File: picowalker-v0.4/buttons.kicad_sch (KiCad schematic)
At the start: 0 parts

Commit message: v0.4: schematic laid out first draft
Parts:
- added C17, C18, C19: 0.1u, Capacitor_SMD:C_0402_1005Metric, symbol Device:C
- added R10, R11, R9: 5.1k, Resistor_SMD:R_0402_1005Metric, symbol Device:R
- added R12, R13, R14: 1k, Resistor_SMD:R_0402_1005Metric, symbol Device:R
- added SW3: BUT_R, symbol Switch:SW_Push
- added SW4: BUT_M, symbol Switch:SW_Push
- added SW5: BUT_L, symbol Switch:SW_Push
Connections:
- new net +3.3V: R10.2, R11.2, R9.2
- new net BUT.L: C19.1, R14.1
- new net BUT.M: C18.1, R13.1
- new net BUT.R: C17.1, R12.1
- new net BUT_L_1: R11.1, R14.2, SW5.2
- new net BUT_M_1: R10.1, R13.2, SW4.2
- new net BUT_R_1: R12.2, R9.1, SW3.2
- new net GND: C17.2, C18.2, C19.2, SW3.1, SW4.1, SW5.1
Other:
- note added: "Press resistor"
- note added: "Release resistor"

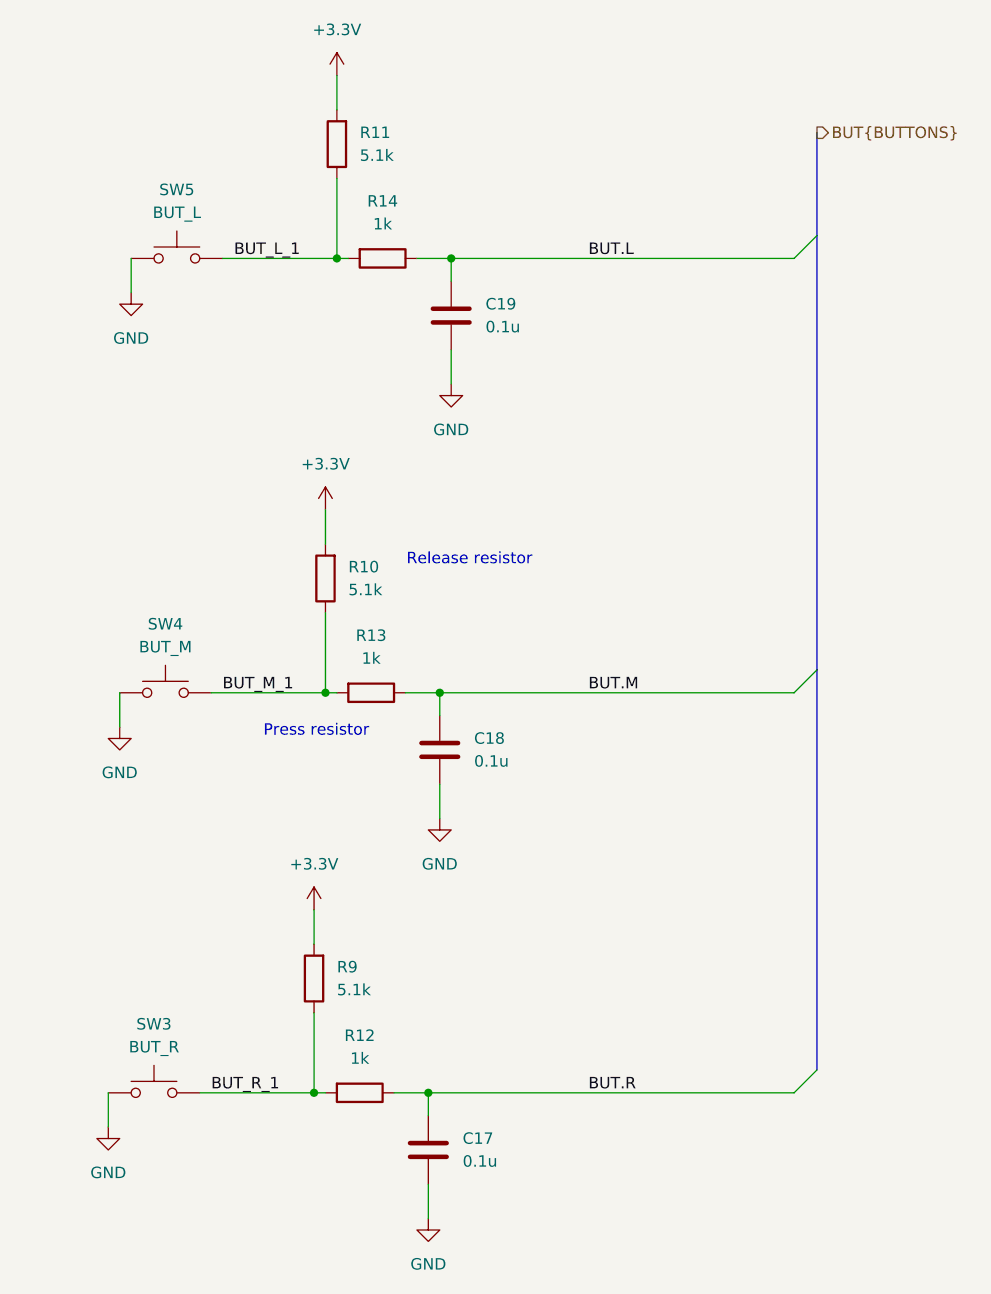
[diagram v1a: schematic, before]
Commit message: v0.4: first rough placement of PCB
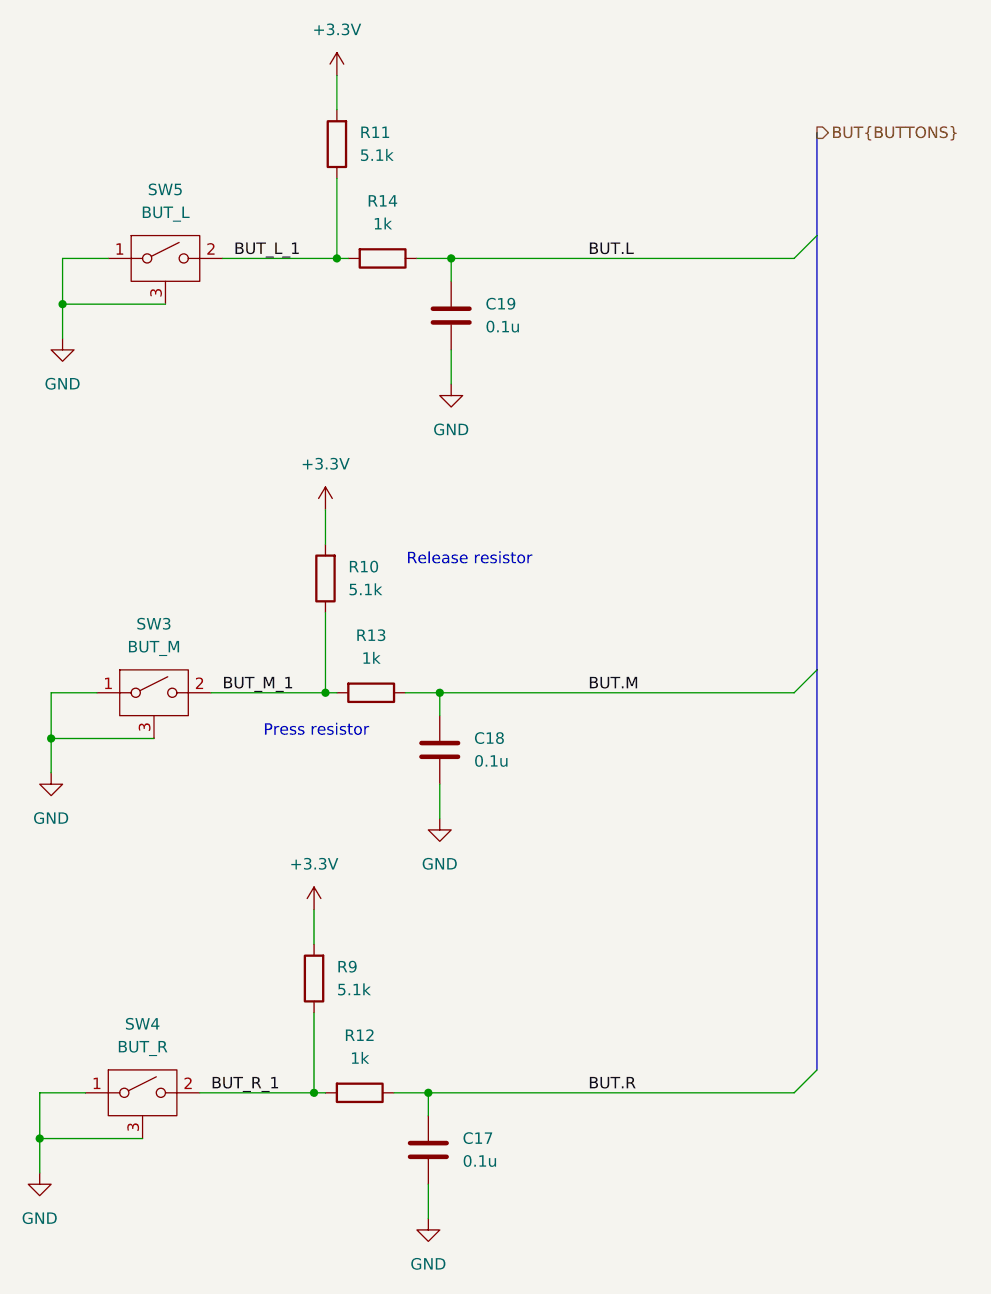
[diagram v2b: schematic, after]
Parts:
- removed SW3: BUT_R, symbol Switch:SW_Push
- removed SW4: BUT_M, symbol Switch:SW_Push
- removed SW5: BUT_L, symbol Switch:SW_Push
- added SW3: BUT_M, picowalker:Button_membrane_4.2mm, symbol picowalker:SW_SPST_Shield
- added SW4: BUT_R, picowalker:Button_membrane_4.2mm, symbol picowalker:SW_SPST_Shield
- added SW5: BUT_L, picowalker:Button_membrane_4.2mm, symbol picowalker:SW_SPST_Shield
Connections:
- net BUT_L_1: now also SW5.2 (B)
- net BUT_M_1: now also SW3.2 (B)
- net BUT_R_1: now also SW4.2 (B)
- net GND: now also SW3.1 (A), SW3.3 (SHIELD), SW4.1 (A), SW4.3 (SHIELD), SW5.1 (A), SW5.3 (SHIELD)

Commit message: v0.4: good start on routing
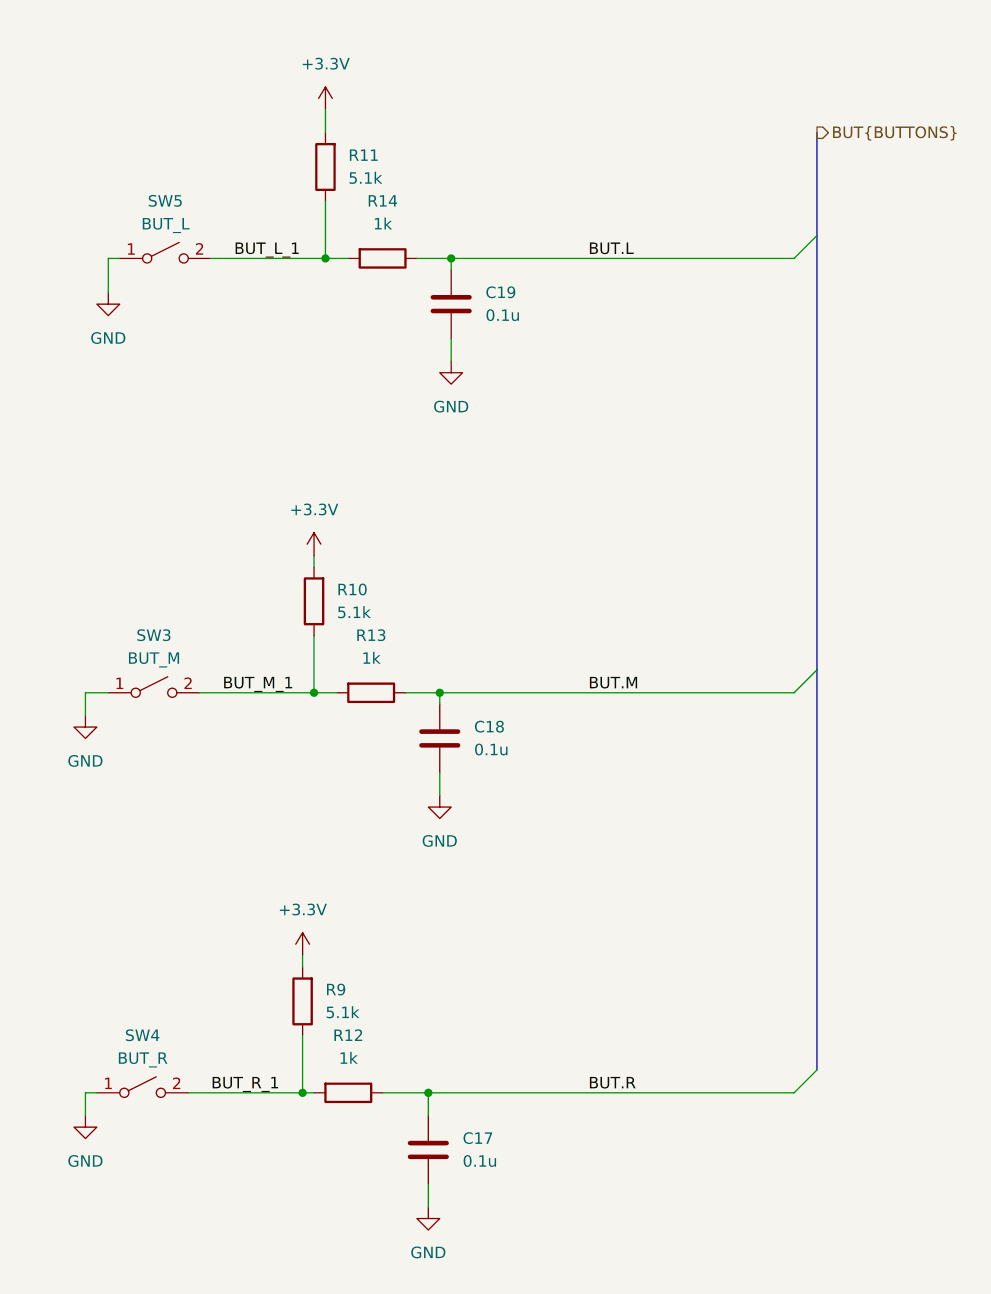
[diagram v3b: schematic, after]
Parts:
- SW3, SW4, SW5: symbol picowalker:SW_SPST_Shield -> Switch:SW_SPST
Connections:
- net GND: no longer SW3.3 (SHIELD), SW4.3 (SHIELD), SW5.3 (SHIELD)
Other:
- note removed: "Press resistor"
- note removed: "Release resistor"
- moved on the sheet: C18, C19, R10, R11, R12, R9

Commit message: v0.4: drc mostly done, need to fiddle with TH1
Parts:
- SW3, SW4, SW5: now left out of the parts list
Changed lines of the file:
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@@
 		(unit 1)
 		(exclude_from_sim no)
-		(in_bom yes)
+		(in_bom no)
 		(on_board yes)
 		(dnp no)
@@
 		(unit 1)
 		(exclude_from_sim no)
-		(in_bom yes)
+		(in_bom no)
 		(on_board yes)
 		(dnp no)
@@
 		(unit 1)
 		(exclude_from_sim no)
-		(in_bom yes)
-		(on_board yes)
-		(dnp no)
+		(in_bom no)
+		(on_board yes)
+		(dnp no)
